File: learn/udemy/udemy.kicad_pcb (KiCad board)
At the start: 2 copper layers, 50.6 x 28.1 mm, 13 parts, among them J1 Screw_Terminal_01x02, J2 Screw_Terminal_01x02, J3 Screw_Terminal_01x02, U1 L7809, U2 L7805

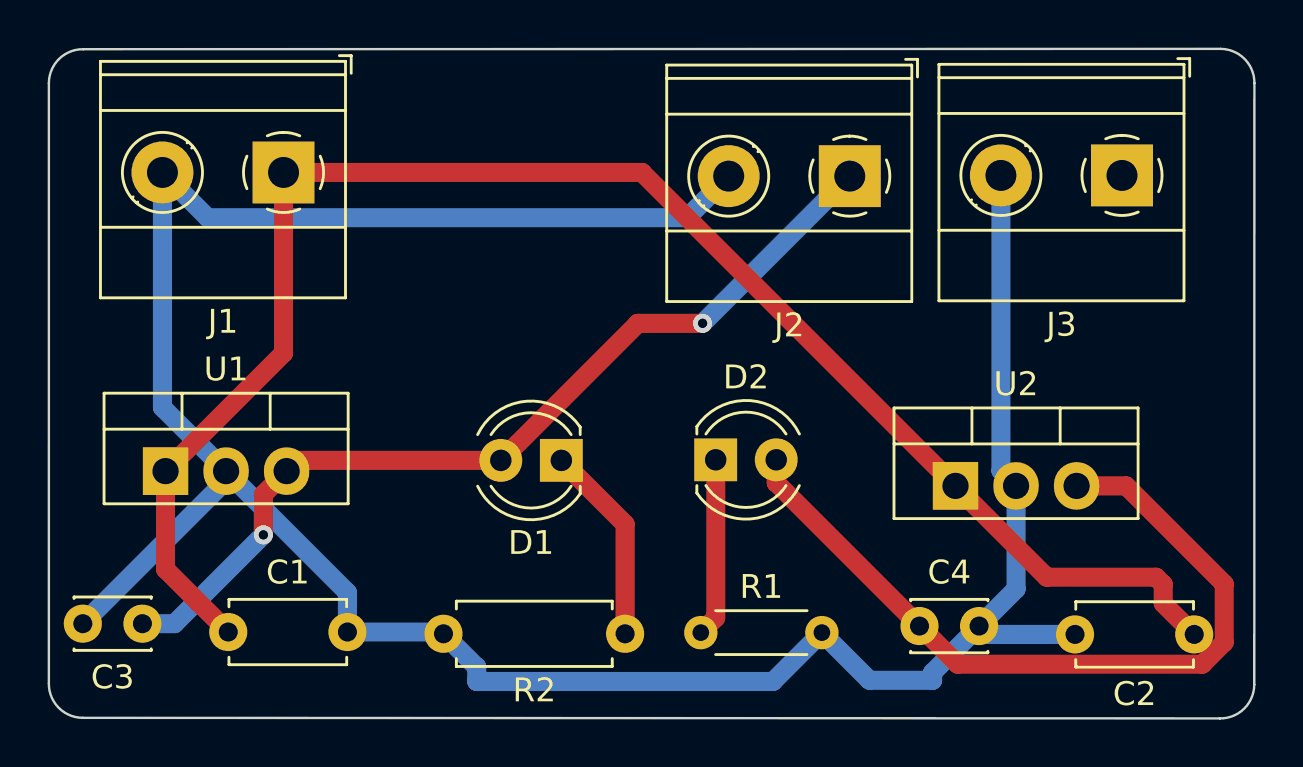
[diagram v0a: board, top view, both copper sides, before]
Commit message: 18/01/23 correzione PCB
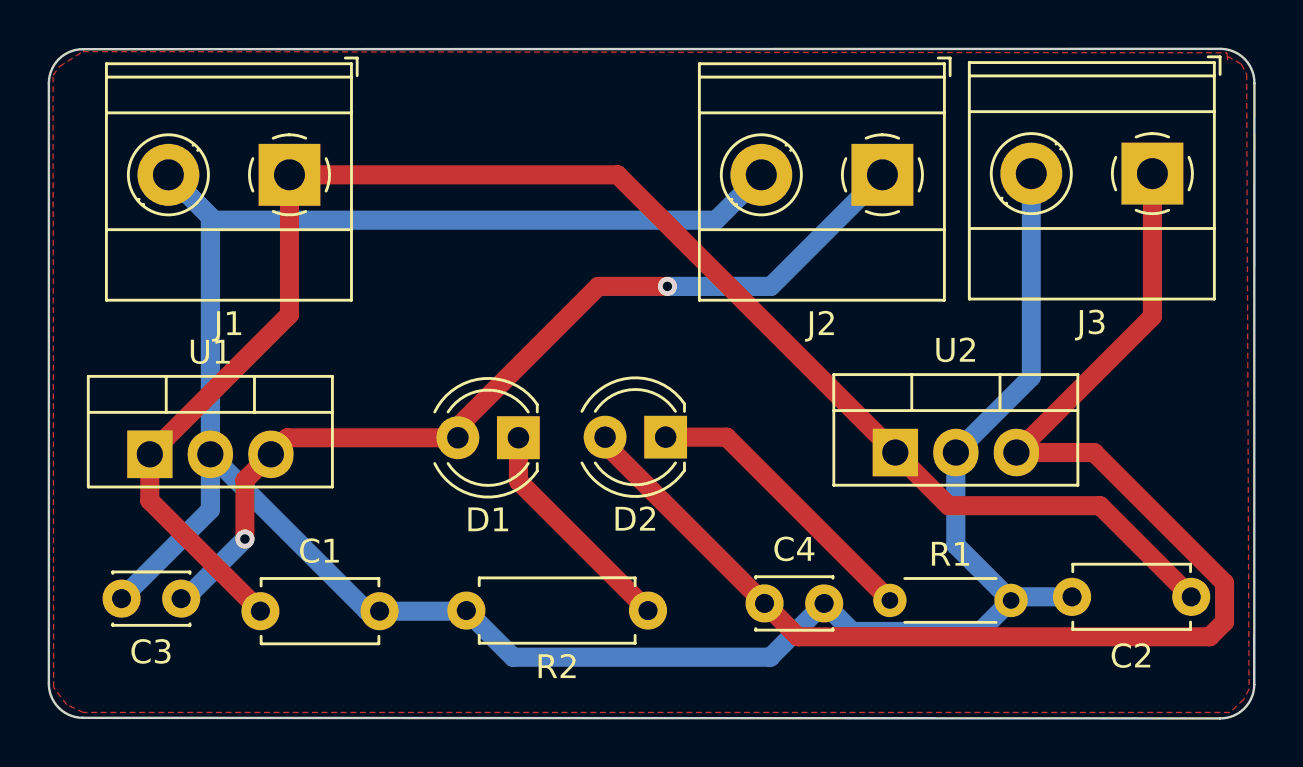
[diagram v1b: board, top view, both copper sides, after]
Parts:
- moved R1 8.05 mm to (151.5, 77.9)
- moved C4 6.57 mm to (146.2, 78.0)
- moved U2 2.89 mm to (151.7, 71.7)
- moved D2 2.30 mm to (142.1, 71.0), turned to 180 degrees
- moved D1 2.04 mm to (135.9, 71.1)
- moved C3 1.93 mm to (121.7, 77.8)
- moved C1 1.61 mm to (125.0, 78.3)
- moved C2 1.58 mm to (164.1, 77.8)
- moved J2 1.37 mm to (151.1, 60.0)
- moved R2 1.37 mm to (141.3, 78.3)
- moved J3 1.28 mm to (162.5, 60.0)
- moved U1 0.97 mm to (120.4, 71.8)
- moved J1 0.27 mm to (126.3, 60.0)
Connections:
- C1 pad 1: GND -> +12V
- C2 pad 1: GND -> +12V
- C3 pad 1: GND -> /9v out
- C4 pad 1: GND -> /5v out
- D1 pad 2: GND -> /9v out
- D2 pad 2: GND -> /5v out
- J1 pad 1: GND -> +12V
- J2 pad 1: GND -> /9v out
- U1 pad 1: GND -> +12V
- U1 pad 3: GND -> /9v out
- U2 pad 1: GND -> +12V
- U2 pad 3: GND -> /5v out
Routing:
- net GND: track 255.1 -> 108.4 mm, vias 2 -> 0
- net +12V: track 0.00 -> 67.8 mm
- net /5v out: track 0.00 -> 56.6 mm
- net /9v out: track 0.00 -> 38.5 mm, vias 0 -> 2
- net Net-(D2-Pad1): track 7.51 -> 12.2 mm
- net Net-(D1-Pad1): track 8.38 -> 9.50 mm
- added copper zone on F.Cu, net (none)
